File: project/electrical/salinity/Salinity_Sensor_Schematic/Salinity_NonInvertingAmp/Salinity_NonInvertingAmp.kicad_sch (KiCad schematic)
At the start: 13 parts, among them U1 MCP6L01, U2 MCP6L01, U3 MCP6L01

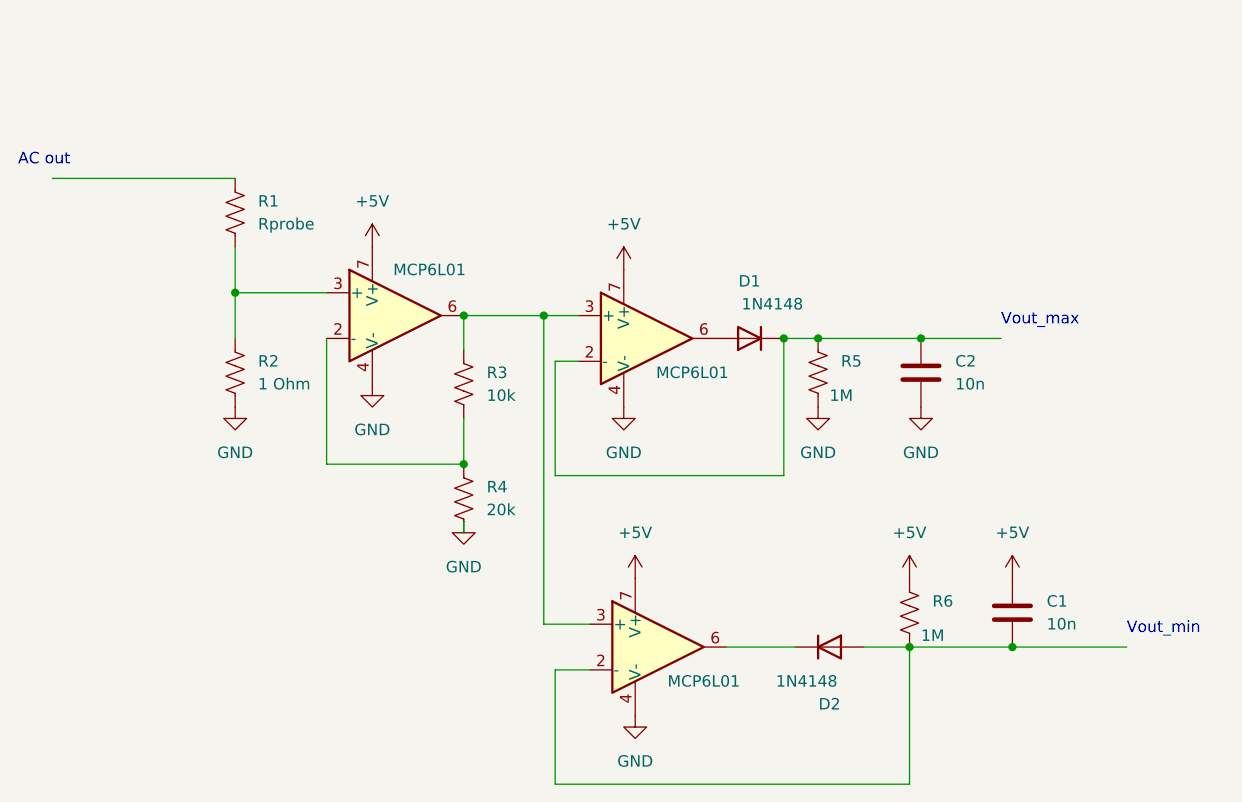
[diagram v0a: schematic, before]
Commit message: Made some circuits better for overleaf
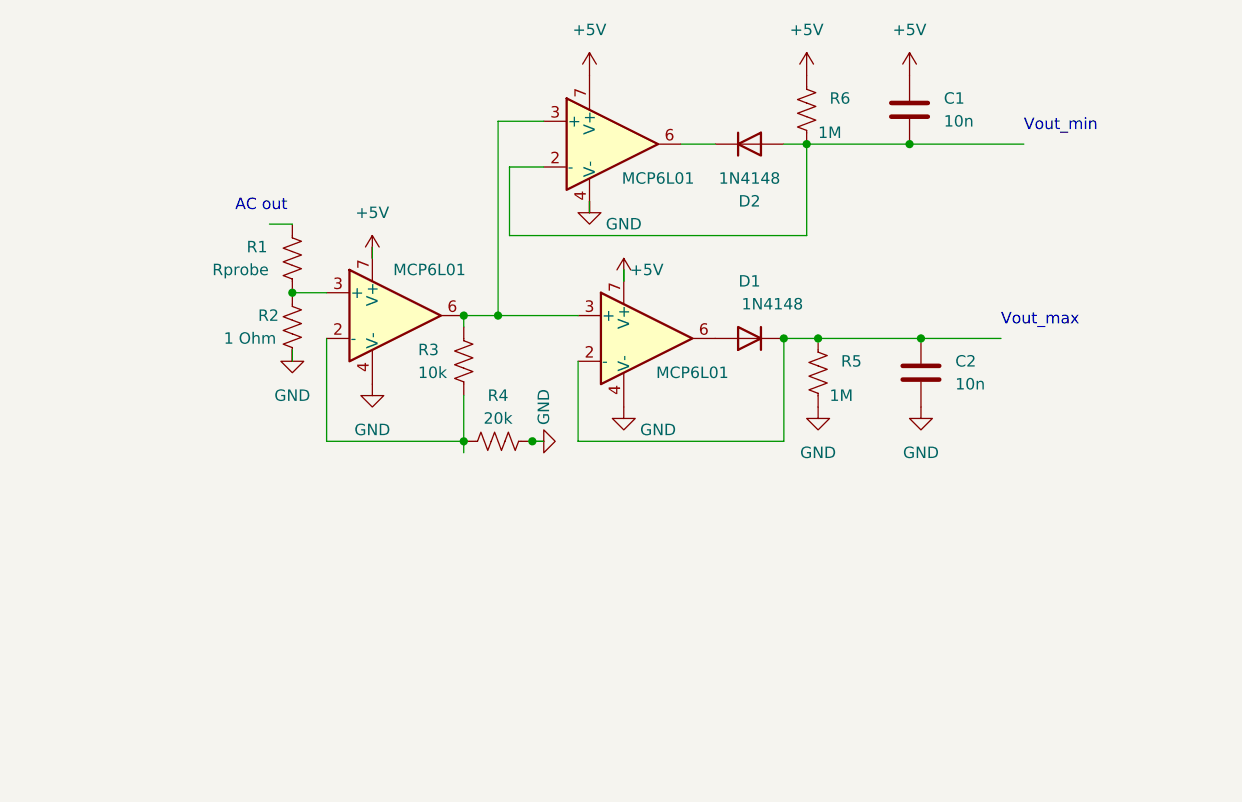
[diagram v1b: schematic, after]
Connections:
- net GND: now also R4.1; no longer R4.2
- net at R3.2, U1.2 (-): now also R4.2; no longer R4.1
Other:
- moved on the sheet: C1, D2, R1, R2, R3, R4, R6
